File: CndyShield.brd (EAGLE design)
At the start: 69.9 x 78.1 mm, 36 parts, among them U1 ARDUINOR3-BPLACE

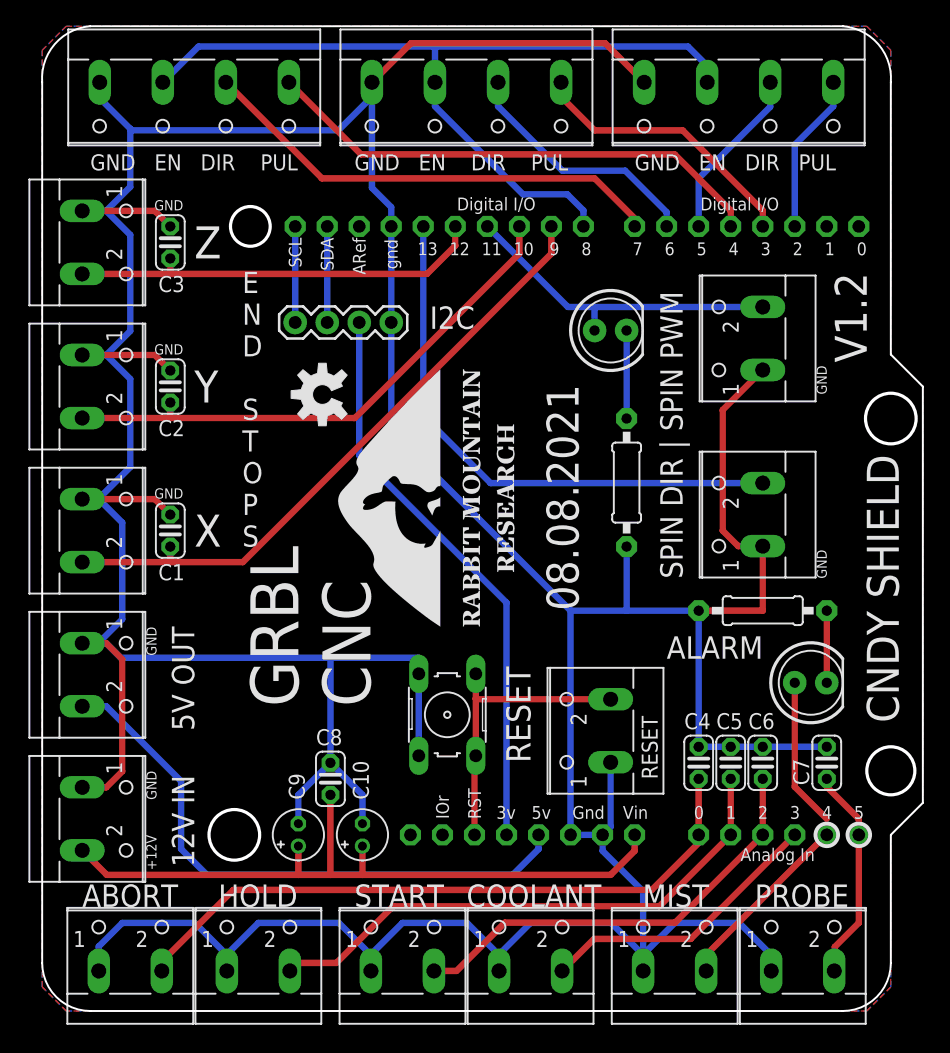
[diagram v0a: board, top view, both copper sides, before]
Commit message: Add files via upload
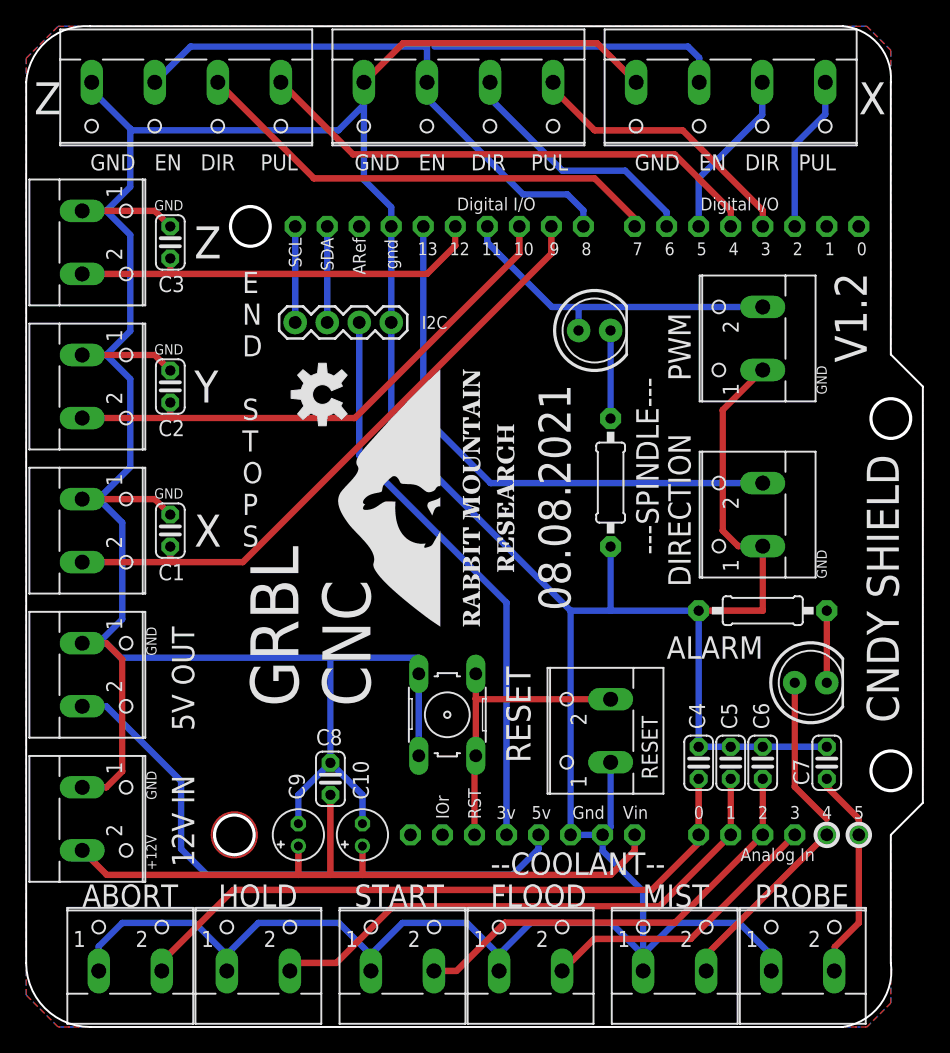
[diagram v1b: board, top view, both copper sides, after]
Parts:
- moved R2 1.27 mm to (80.6, 53.3)
- moved D2 1.27 mm to (79.4, 65.4)
- moved X 0.64 mm to (90.2, 83.8)
- moved Y 0.64 mm to (68.6, 83.8)
- moved Z 0.63 mm to (47.0, 83.8)
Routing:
- net SPIN_E: track 26.4 -> 27.1 mm
- net N$6: track 40.5 -> 41.2 mm
- net N$5: track 37.5 -> 38.2 mm
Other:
- board size 69.9 x 78.1 mm -> 71.1 x 79.4 mm
- board text added: "---SPINDLE---"
- board text added: "--COOLANT--"
- board text added: "DIRECTION PWM"
- board text added: "FLOOD"
- board text removed: "COOLANT"
- board text removed: "SPIN DIR | SPIN PWM"
